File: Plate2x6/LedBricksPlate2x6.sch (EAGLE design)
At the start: 8 parts, among them J1 SM02B-SRSS-TB, J2 SM02B-SRSS-TB

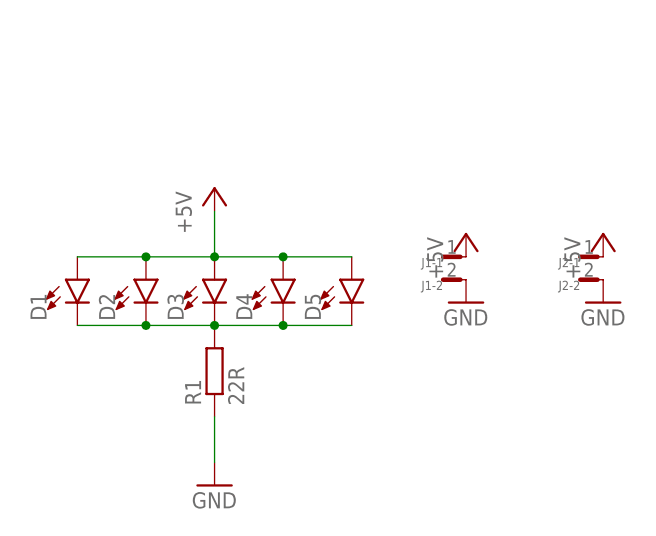
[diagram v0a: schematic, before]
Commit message: gerbers, pnp file
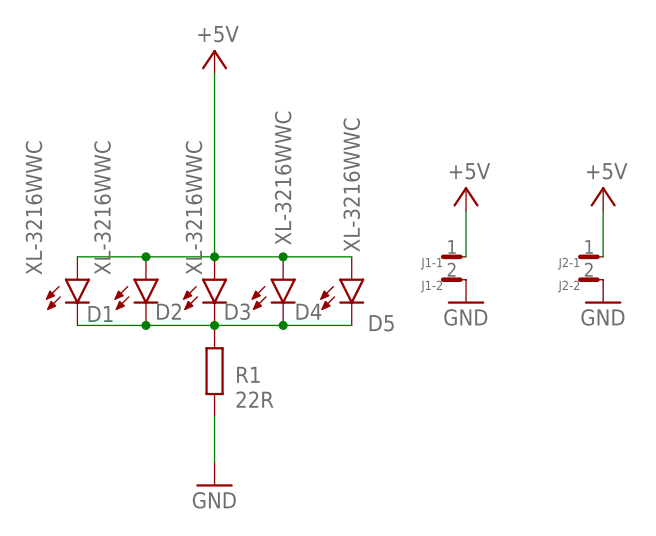
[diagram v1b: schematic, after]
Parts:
- D1, D2, D3, D4, D5: value (none) -> XL-3216WWC
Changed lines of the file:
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@@
 </classes>
 <parts>
-<part name="D1" library="SparkFun-LED" library_urn="urn:adsk.eagle:library:529" deviceset="LED" device="1206" package3d_urn="urn:adsk.eagle:package:39352/1"/>
-<part name="D2" library="SparkFun-LED" library_urn="urn:adsk.eagle:library:529" deviceset="LED" device="1206" package3d_urn="urn:adsk.eagle:package:39352/1"/>
-<part name="D3" library="SparkFun-LED" library_urn="urn:adsk.eagle:library:529" deviceset="LED" device="1206" package3d_urn="urn:adsk.eagle:package:39352/1"/>
-<part name="D4" library="SparkFun-LED" library_urn="urn:adsk.eagle:library:529" deviceset="LED" device="1206" package3d_urn="urn:adsk.eagle:package:39352/1"/>
-<part name="D5" library="SparkFun-LED" library_urn="urn:adsk.eagle:library:529" deviceset="LED" device="1206" package3d_urn="urn:adsk.eagle:package:39352/1"/>
+<part name="D1" library="SparkFun-LED" library_urn="urn:adsk.eagle:library:529" deviceset="LED" device="1206" package3d_urn="urn:adsk.eagle:package:39352/1" value="XL-3216WWC"/>
+<part name="D2" library="SparkFun-LED" library_urn="urn:adsk.eagle:library:529" deviceset="LED" device="1206" package3d_urn="urn:adsk.eagle:package:39352/1" value="XL-3216WWC"/>
+<part name="D3" library="SparkFun-LED" library_urn="urn:adsk.eagle:library:529" deviceset="LED" device="1206" package3d_urn="urn:adsk.eagle:package:39352/1" value="XL-3216WWC"/>
+<part name="D4" library="SparkFun-LED" library_urn="urn:adsk.eagle:library:529" deviceset="LED" device="1206" package3d_urn="urn:adsk.eagle:package:39352/1" value="XL-3216WWC"/>
+<part name="D5" library="SparkFun-LED" library_urn="urn:adsk.eagle:library:529" deviceset="LED" device="1206" package3d_urn="urn:adsk.eagle:package:39352/1" value="XL-3216WWC"/>
 <part name="R1" library="resistor" library_urn="urn:adsk.eagle:library:348" deviceset="R-EU_" device="R0805" package3d_urn="urn:adsk.eagle:package:23553/2" value="22R"/>
 <part name="P+1" library="supply1" library_urn="urn:adsk.eagle:library:371" deviceset="+5V" device=""/>
@@
 <instances>
 <instance part="D1" gate="G$1" x="2.54" y="0" smashed="yes">
-<attribute name="NAME" x="-0.889" y="-4.572" size="1.778" layer="95" font="vector" rot="R90"/>
-<attribute name="VALUE" x="4.445" y="-4.572" size="1.778" layer="96" font="vector" rot="R90" align="top-left"/>
+<attribute name="NAME" x="3.556" y="-4.699" size="1.778" layer="95" font="vector"/>
+<attribute name="VALUE" x="-3.175" y="0.508" size="1.778" layer="96" font="vector" rot="R90" align="top-left"/>
 </instance>
 <instance part="D2" gate="G$1" x="10.16" y="0" smashed="yes">
-<attribute name="NAME" x="6.731" y="-4.572" size="1.778" layer="95" font="vector" rot="R90"/>
-<attribute name="VALUE" x="12.065" y="-4.572" size="1.778" layer="96" font="vector" rot="R90" align="top-left"/>
+<attribute name="NAME" x="11.176" y="-4.445" size="1.778" layer="95" font="vector"/>
+<attribute name="VALUE" x="4.445" y="0.508" size="1.778" layer="96" font="vector" rot="R90" align="top-left"/>
 </instance>
 <instance part="D3" gate="G$1" x="17.78" y="0" smashed="yes">
-<attribute name="NAME" x="14.351" y="-4.572" size="1.778" layer="95" font="vector" rot="R90"/>
-<attribute name="VALUE" x="19.685" y="-4.572" size="1.778" layer="96" font="vector" rot="R90" align="top-left"/>
+<attribute name="NAME" x="18.796" y="-4.445" size="1.778" layer="95" font="vector"/>
+<attribute name="VALUE" x="14.605" y="0.508" size="1.778" layer="96" font="vector" rot="R90" align="top-left"/>
 </instance>
 <instance part="D4" gate="G$1" x="25.4" y="0" smashed="yes">
-<attribute name="NAME" x="21.971" y="-4.572" size="1.778" layer="95" font="vector" rot="R90"/>
-<attribute name="VALUE" x="27.305" y="-4.572" size="1.778" layer="96" font="vector" rot="R90" align="top-left"/>
+<attribute name="NAME" x="26.67" y="-4.445" size="1.778" layer="95" font="vector"/>
+<attribute name="VALUE" x="24.511" y="3.81" size="1.778" layer="96" font="vector" rot="R90" align="top-left"/>
 </instance>
 <instance part="D5" gate="G$1" x="33.02" y="0" smashed="yes">
-<attribute name="NAME" x="29.591" y="-4.572" size="1.778" layer="95" font="vector" rot="R90"/>
-<attribute name="VALUE" x="34.925" y="-4.572" size="1.778" layer="96" font="vector" rot="R90" align="top-left"/>
+<attribute name="NAME" x="34.798" y="-5.715" size="1.778" layer="95" font="vector"/>
+<attribute name="VALUE" x="32.131" y="3.048" size="1.778" layer="96" font="vector" rot="R90" align="top-left"/>
 </instance>
 <instance part="R1" gate="G$1" x="17.78" y="-10.16" smashed="yes" rot="R90">
-<attribute name="NAME" x="16.2814" y="-13.97" size="1.778" layer="95" rot="R90"/>
-<attribute name="VALUE" x="21.082" y="-13.97" size="1.778" layer="96" rot="R90"/>
+<attribute name="NAME" x="20.066" y="-11.4554" size="1.778" layer="95"/>
+<attribute name="VALUE" x="20.066" y="-14.224" size="1.778" layer="96"/>
 </instance>
-<instance part="P+1" gate="1" x="17.78" y="10.16" smashed="yes">
-<attribute name="VALUE" x="15.24" y="5.08" size="1.778" layer="96" rot="R90"/>
+<instance part="P+1" gate="1" x="17.78" y="25.4" smashed="yes">
+<attribute name="VALUE" x="15.748" y="26.416" size="1.778" layer="96"/>
 </instance>
 <instance part="GND1" gate="1" x="17.78" y="-22.86" smashed="yes">
@@
 <attribute name="VALUE" x="58.42" y="-5.08" size="1.778" layer="96"/>
 </instance>
-<instance part="P+2" gate="1" x="45.72" y="5.08" smashed="yes">
-<attribute name="VALUE" x="43.18" y="0" size="1.778" layer="96" rot="R90"/>
+<instance part="P+2" gate="1" x="45.72" y="10.16" smashed="yes">
+<attribute name="VALUE" x="43.688" y="11.176" size="1.778" layer="96"/>
 </instance>
 <instance part="J1" gate="-1" x="43.18" y="2.54" smashed="yes">
@@
 <attribute name="NAME" x="58.42" y="-0.635" size="1.016" layer="95" rot="R180" align="center-left"/>
 </instance>
-<instance part="P+3" gate="1" x="60.96" y="5.08" smashed="yes">
-<attribute name="VALUE" x="58.42" y="0" size="1.778" layer="96" rot="R90"/>
+<instance part="P+3" gate="1" x="60.96" y="10.16" smashed="yes">
+<attribute name="VALUE" x="58.928" y="11.176" size="1.778" layer="96"/>
 </instance>
 </instances>
@@
 <wire x1="25.4" y1="2.54" x2="33.02" y2="2.54" width="0.1524" layer="91"/>
 <junction x="25.4" y="2.54"/>
-<wire x1="17.78" y1="2.54" x2="17.78" y2="7.62" width="0.1524" layer="91"/>
+<wire x1="17.78" y1="2.54" x2="17.78" y2="22.86" width="0.1524" layer="91"/>
 <pinref part="P+1" gate="1" pin="+5V"/>
 </segment>
@@
 <pinref part="J1" gate="-1" pin="P"/>
 <pinref part="P+2" gate="1" pin="+5V"/>
+<wire x1="45.72" y1="7.62" x2="45.72" y2="2.54" width="0.1524" layer="91"/>
 </segment>
 <segment>
 <pinref part="J2" gate="-1" pin="P"/>
 <pinref part="P+3" gate="1" pin="+5V"/>
+<wire x1="60.96" y1="7.62" x2="60.96" y2="2.54" width="0.1524" layer="91"/>
 </segment>
 </net>
